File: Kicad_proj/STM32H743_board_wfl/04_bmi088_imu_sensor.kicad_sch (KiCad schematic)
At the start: 5 parts, among them U5 BMI088

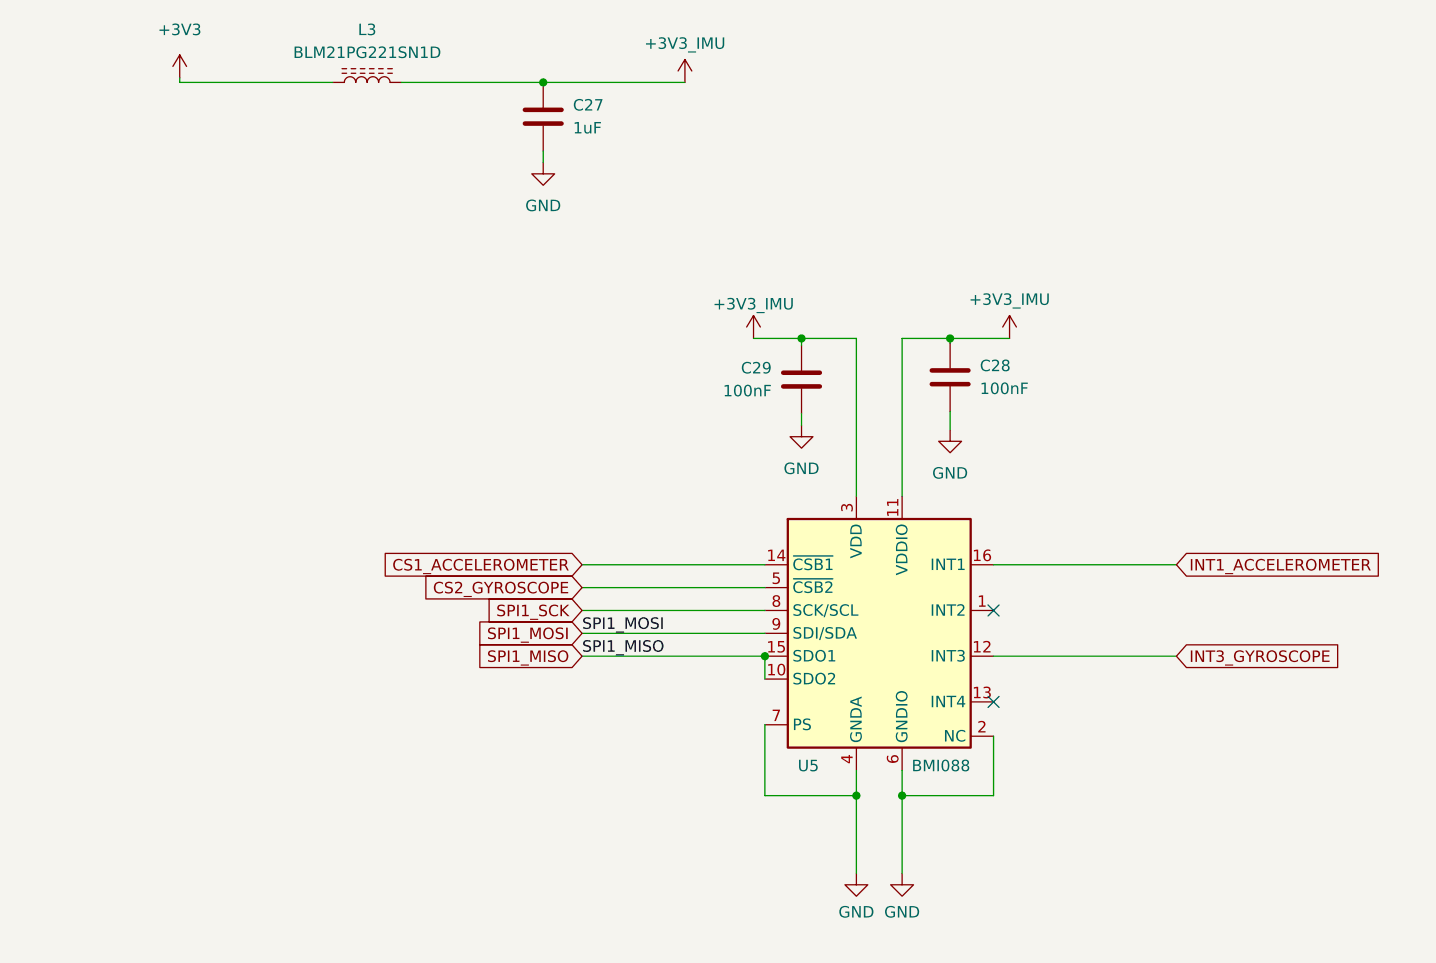
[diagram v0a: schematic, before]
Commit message: v0.5 schematics + lib update
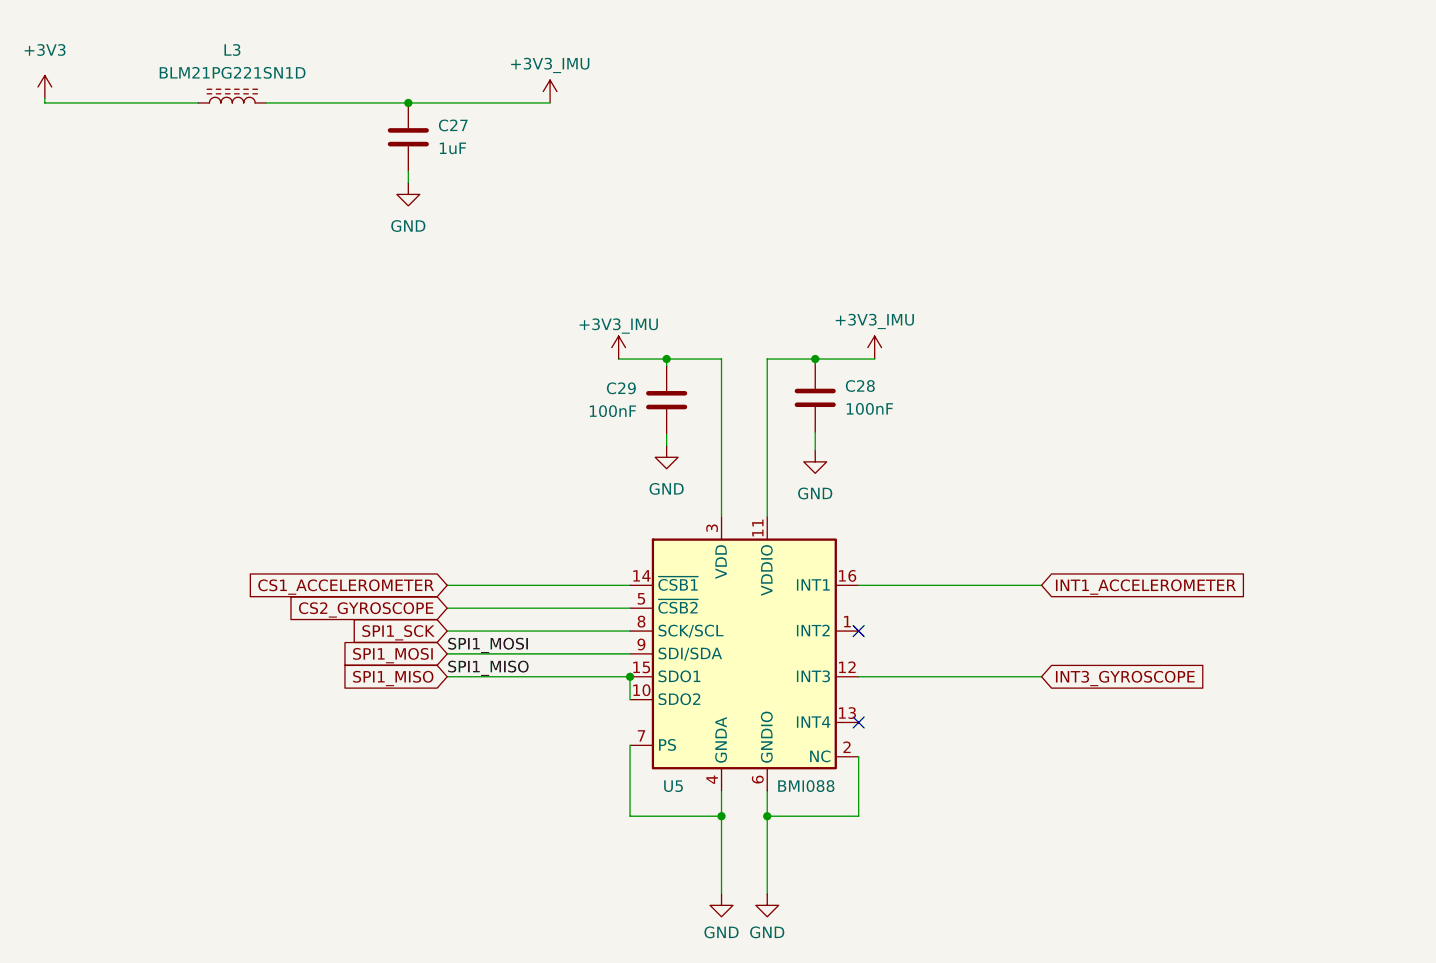
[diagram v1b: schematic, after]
